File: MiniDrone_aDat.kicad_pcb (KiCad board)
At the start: 2 copper layers, 50 parts, among them J1 Screw_Terminal_01x02, J10 Conn_01x04, J2 Screw_Terminal_01x02, J3 Screw_Terminal_01x02, J4 Screw_Terminal_01x02, J5 Screw_Terminal_01x02, J6 Conn_01x08, J7 Conn_01x04, J8 Conn_02x04_Counter_Clockwise, J9 Conn_01x04, SW1 SW_Push, U1 STM32F103C8Tx, U2 ADP7142AUJZ-3.3, U3 MX1508, U4 MCP601-xOT, U5 MX1508, Y1 5032 2P

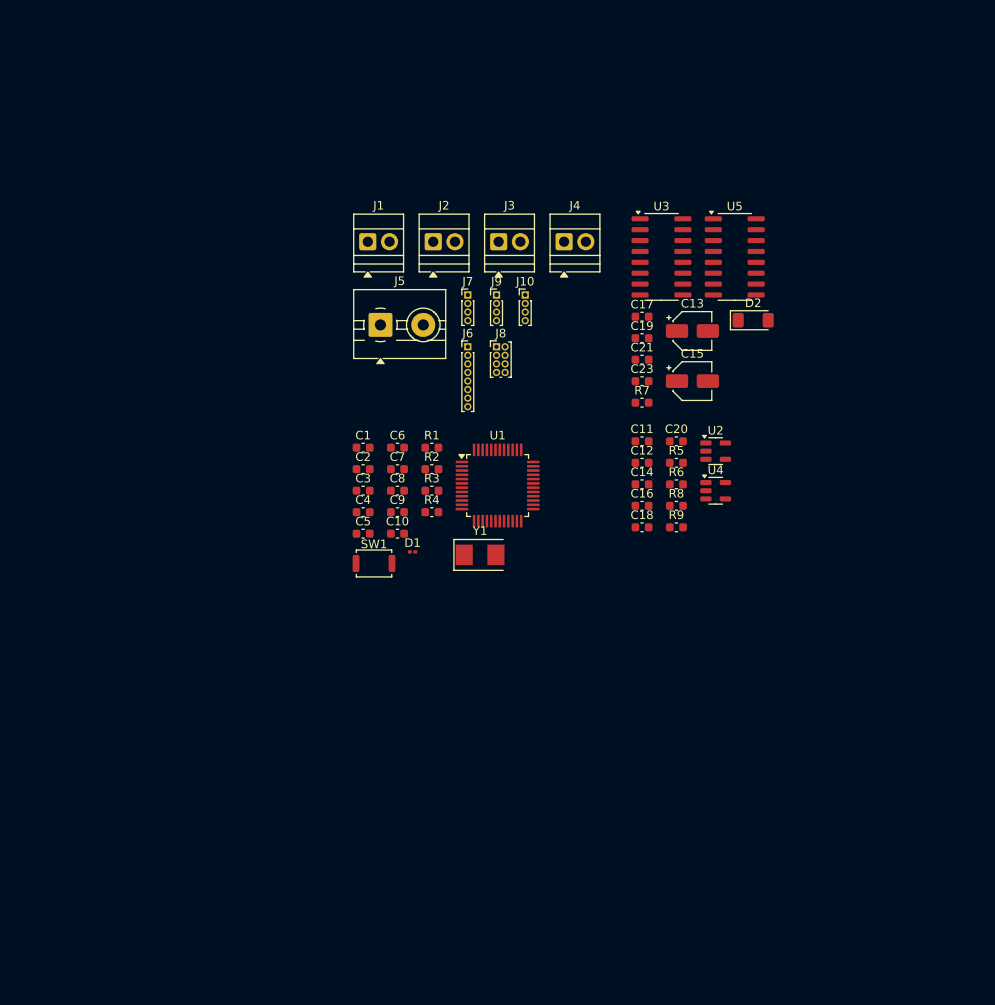
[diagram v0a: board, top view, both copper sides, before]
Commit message: 2/7/2025
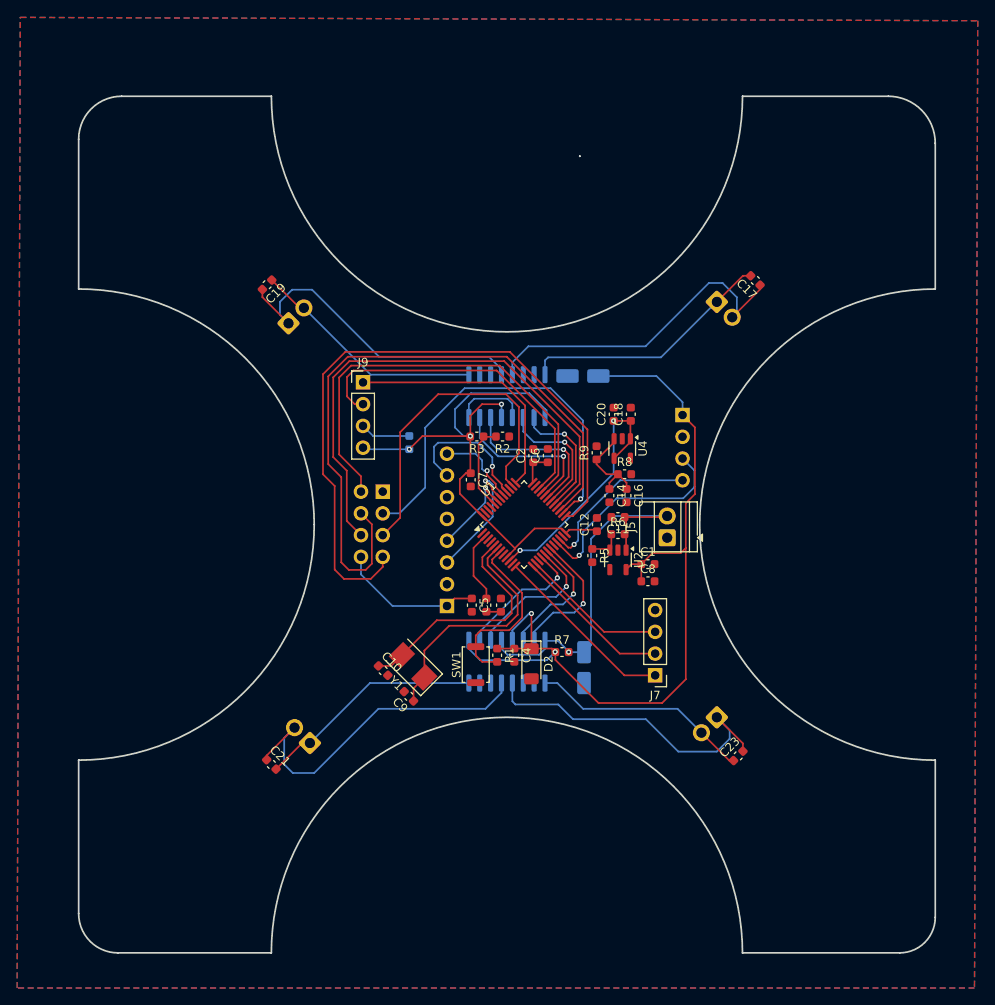
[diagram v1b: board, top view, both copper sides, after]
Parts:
- C13, C15, C3, J1, J2, J3, J4, U3, U5: moved to B.Cu
- D1: footprint Capacitor_SMD:C_0201_0603Metric -> Capacitor_SMD:C_0603_1608Metric
- J10: footprint Connector_PinHeader_1.00mm:PinHeader_1x04_P1.00mm_Vertical -> Connector_PinHeader_2.54mm:PinHeader_1x04_P2.54mm_Vertical; moved to B.Cu
- J5: footprint TerminalBlock:TerminalBlock_MaiXu_MX126-5.0-02P_1x02_P5.00mm -> TerminalBlock:TerminalBlock_Xinya_XY308-2.54-2P_1x02_P2.54mm_Horizontal
- J6: footprint Connector_PinHeader_1.00mm:PinHeader_1x08_P1.00mm_Vertical -> Connector_PinHeader_2.54mm:PinHeader_1x08_P2.54mm_Vertical; moved to B.Cu
- J7, J9: footprint Connector_PinHeader_1.00mm:PinHeader_1x04_P1.00mm_Vertical -> Connector_PinHeader_2.54mm:PinHeader_1x04_P2.54mm_Vertical
- J8: footprint Connector_PinHeader_1.00mm:PinHeader_2x04_P1.00mm_Vertical -> Connector_PinHeader_2.54mm:PinHeader_2x04_P2.54mm_Vertical; moved to B.Cu
- moved J4 65.6 mm to (77.0, 125.5), turned to 135 degrees
- moved C21 64.1 mm to (72.5, 128.0), turned to -45 degrees
- moved J3 61.1 mm to (124.5, 122.5), turned to -135 degrees
- moved U3 50.6 mm to (100.0, 116.0), turned to -90 degrees
- moved J7 49.5 mm to (117.3, 117.6), turned to 180 degrees
- moved D2 47.7 mm to (102.9, 116.2), turned to -90 degrees
- moved C23 45.2 mm to (127.0, 127.0), turned to 45 degrees
- moved C19 44.2 mm to (72.0, 72.0), turned to -135 degrees
- moved J5 41.7 mm to (118.7, 101.5), turned to 90 degrees
- moved J1 41.3 mm to (124.5, 74.0), turned to -45 degrees
- moved C1 35.9 mm to (116.5, 104.6)
- moved C15 35.8 mm to (109.0, 116.7), turned to -90 degrees
- moved U5 31.2 mm to (100.0, 85.0), turned to 90 degrees
- moved C8 31.1 mm to (116.5, 106.6)
- moved R7 30.6 mm to (106.4, 114.9)
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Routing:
- net +3V3: track 0.00 -> 190.4 mm, vias 0 -> 5
- net /TopLevelDesign/PB12: track 0.00 -> 78.5 mm
- net /TopLevelDesign/PB14: track 0.00 -> 77.5 mm
- net /TopLevelDesign/PB15: track 0.00 -> 62.3 mm
- net Vin: track 0.00 -> 54.4 mm, vias 0 -> 1
- net /TopLevelDesign/PA12: track 0.00 -> 52.1 mm
- net /TopLevelDesign/PB13: track 0.00 -> 47.1 mm, vias 0 -> 1
- net /TopLevelDesign/HBridge/H2_OUTB1: track 0.00 -> 40.7 mm
- net /TopLevelDesign/HBridge/H1_OUTB1: track 0.00 -> 39.8 mm
- net /TopLevelDesign/SWDIO: track 0.00 -> 39.7 mm
- net /TopLevelDesign/PA15: track 0.00 -> 39.3 mm
- net /TopLevelDesign/HBridge/H1_OUTA2: track 0.00 -> 39.1 mm
- net /TopLevelDesign/HBridge/H2_OUTA2: track 0.00 -> 38.9 mm
- net /TopLevelDesign/HBridge/H1_OUTA1: track 0.00 -> 29.8 mm
- net /TopLevelDesign/MCU/PA0: track 0.00 -> 29.7 mm, vias 0 -> 2
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- added copper zone on B.Cu, net GND
- added copper zone on F.Cu, net GND
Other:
- board outline added: 100 x 100 mm

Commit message: 4/7/2025
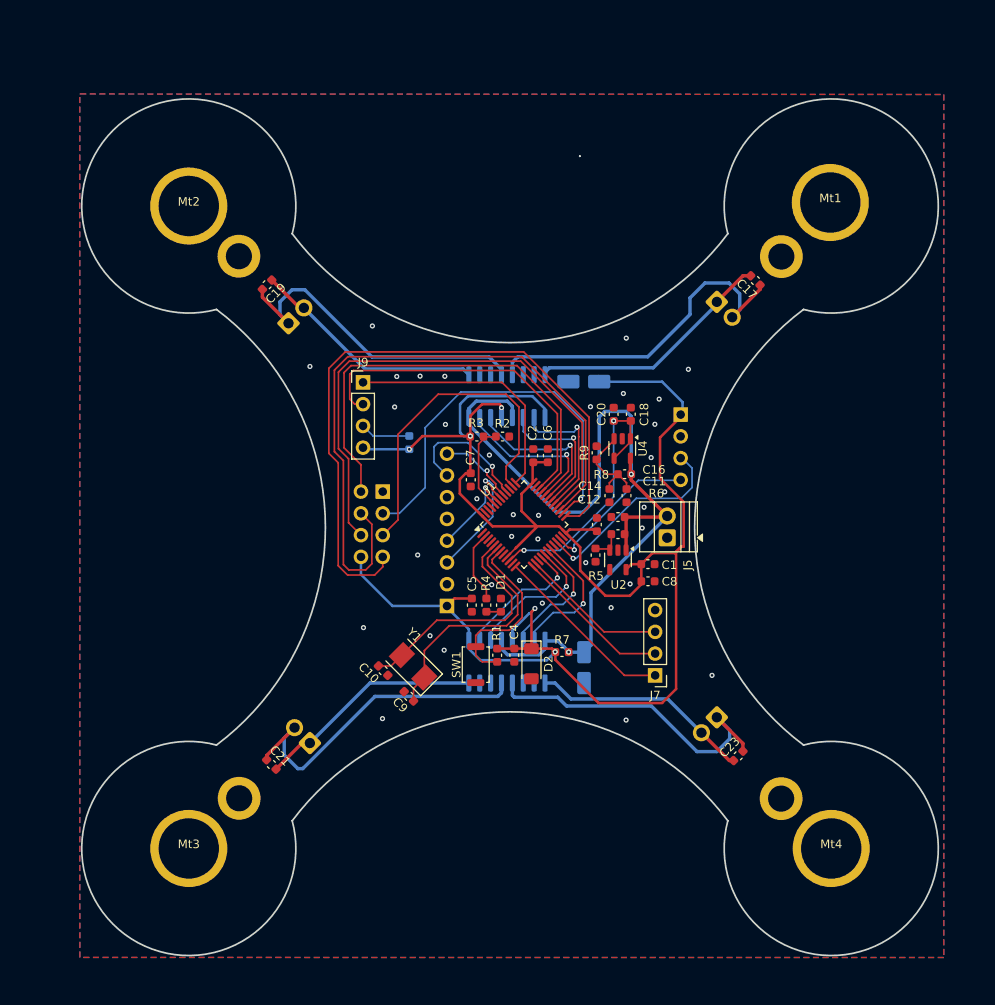
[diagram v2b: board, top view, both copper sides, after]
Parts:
- added Mt1: ~, Motor_Screws:720DCMotor, F.Cu at (137.8, 62.4)
- added Mt2: ~, Motor_Screws:720DCMotor, F.Cu at (62.9, 62.8)
- added Mt3: ~, Motor_Screws:720DCMotor, F.Cu at (62.9, 137.8)
- added Mt4: ~, Motor_Screws:720DCMotor, F.Cu at (137.9, 137.8)
- added Scr1: ~, Motor_Screws:PillarScrew5mmM3, B.Cu at (132.0, 68.7)
- added Scr2: ~, Motor_Screws:PillarScrew5mmM3, B.Cu at (68.7, 68.7)
- added Scr3: ~, Motor_Screws:PillarScrew5mmM3, B.Cu at (132.0, 132.0)
- added Scr4: ~, Motor_Screws:PillarScrew5mmM3, B.Cu at (68.7, 131.9)
- moved C13 0.66 mm to (109.0, 83.3)
- moved R5 0.38 mm to (110.3, 103.6)
- moved J10 0.23 mm to (120.3, 87.2)
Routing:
- net Vin: track 54.4 -> 99.8 mm, vias 1 -> 2
- net +3V3: track 190.4 -> 219.3 mm
- net /TopLevelDesign/HBridge/H1_INA1: track 14.8 -> 17.0 mm
- net /TopLevelDesign/HBridge/H1_OUTB1: track 39.8 -> 41.7 mm
- net /TopLevelDesign/MCU/PA0: track 29.7 -> 31.3 mm
- net /TopLevelDesign/PB10: track 25.4 -> 23.8 mm
- net /TopLevelDesign/HBridge/H1_INB1: track 15.3 -> 16.6 mm
- net /TopLevelDesign/SWDIO: track 39.7 -> 40.9 mm
- net /TopLevelDesign/HBridge/H2_OUTB1: track 40.7 -> 39.6 mm
- net /TopLevelDesign/PA12: track 52.1 -> 53.0 mm
- net /TopLevelDesign/PB15: track 62.3 -> 63.1 mm
- net /TopLevelDesign/PB14: track 77.5 -> 78.2 mm
- net /TopLevelDesign/HBridge/H1_OUTA1: track 29.8 -> 29.1 mm
- net /TopLevelDesign/PB4: track 16.4 -> 15.8 mm
- net /TopLevelDesign/PB11: track 19.2 -> 18.6 mm
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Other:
- outline, holes or cut-outs redrawn
